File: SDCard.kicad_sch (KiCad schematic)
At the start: 1 part, among them J4 Micro_SD_Card_Det

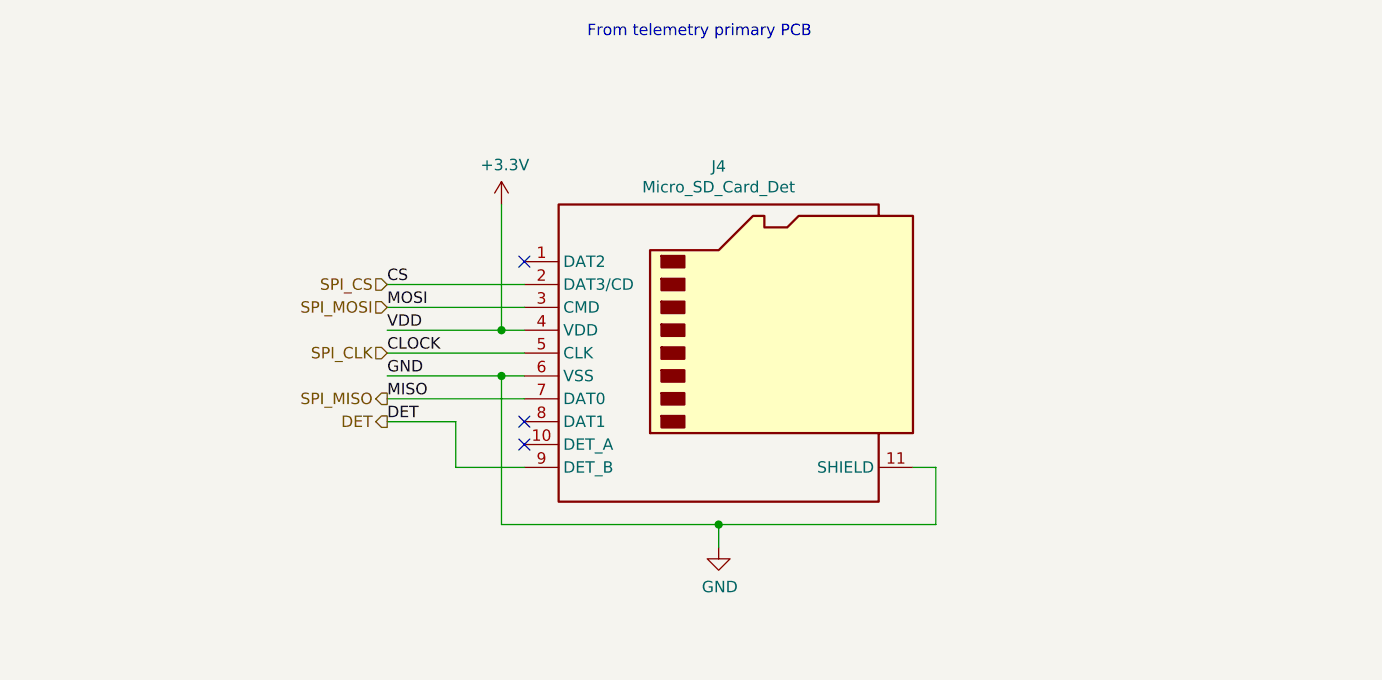
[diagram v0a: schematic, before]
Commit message: Updated pinouts and added protection circuitry for signals
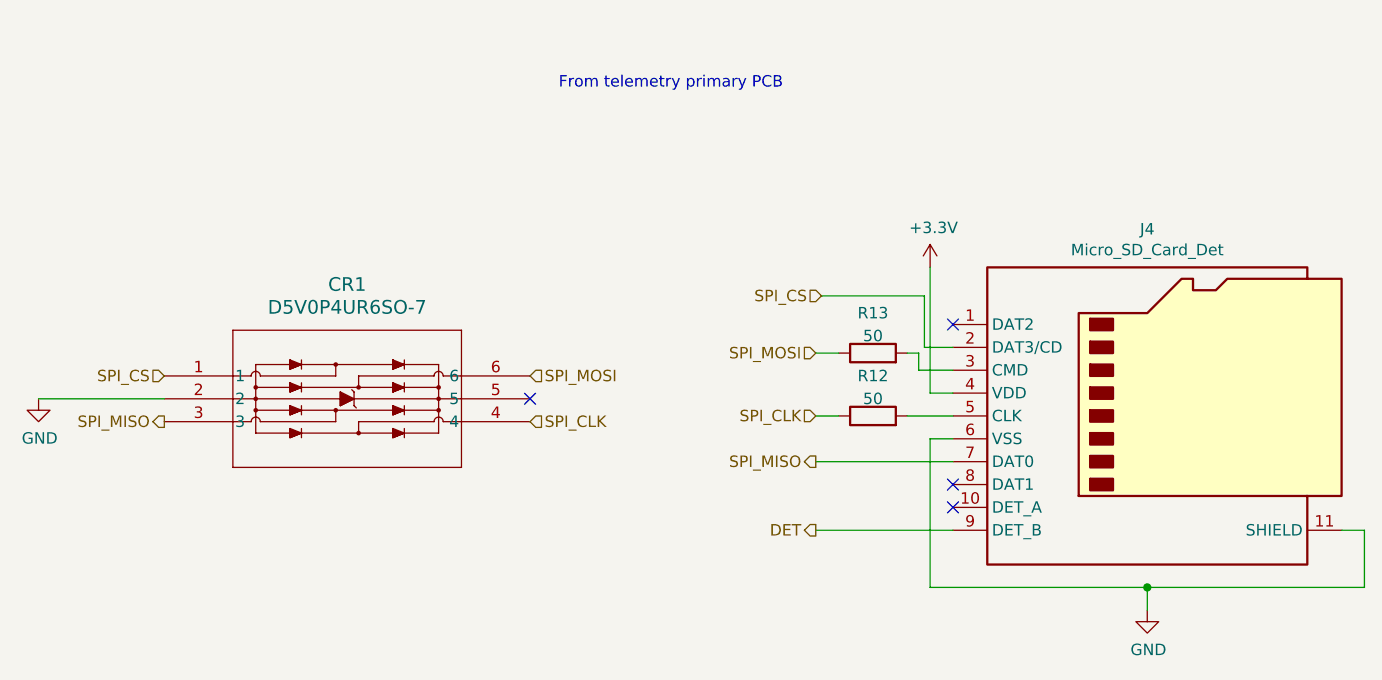
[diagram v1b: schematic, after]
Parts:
- added CR1: D5V0P4UR6SO-7, UTSVT_ICs:SOT26_DIO, symbol utsvt-chips:D5V0P4UR6SO-7
- added R12, R13: 50, Resistor_SMD:R_0805_2012Metric, symbol Device:R
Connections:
- net GND: now also CR1.2
- net SPI_CLK: now also CR1.4, R12.1; no longer J4.5 (CLK)
- net SPI_CS: now also CR1.1
- net SPI_MISO: now also CR1.3
- net SPI_MOSI: now also CR1.6, R13.1; no longer J4.3 (CMD)
- new net: J4.5 (CLK), R12.2
- new net: J4.3 (CMD), R13.2
- no-connect marks 3 -> 4
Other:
- moved on the sheet: J4
